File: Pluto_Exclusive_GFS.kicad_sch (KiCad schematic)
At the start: 26 parts

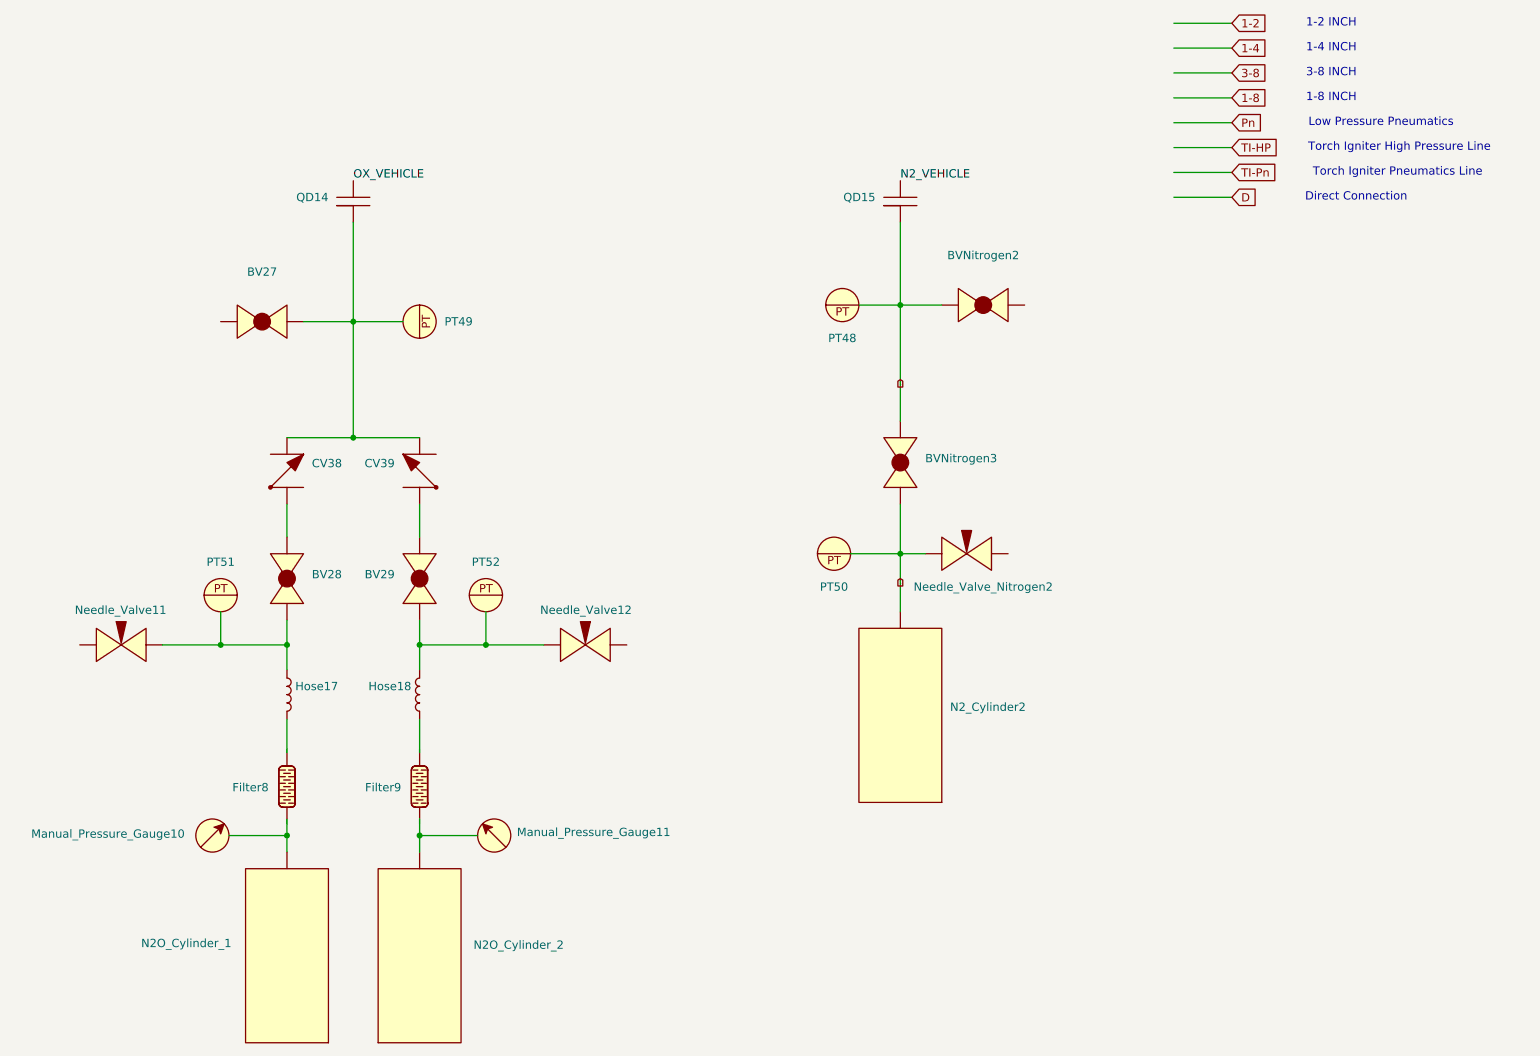
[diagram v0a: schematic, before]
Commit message: more silwood stuff
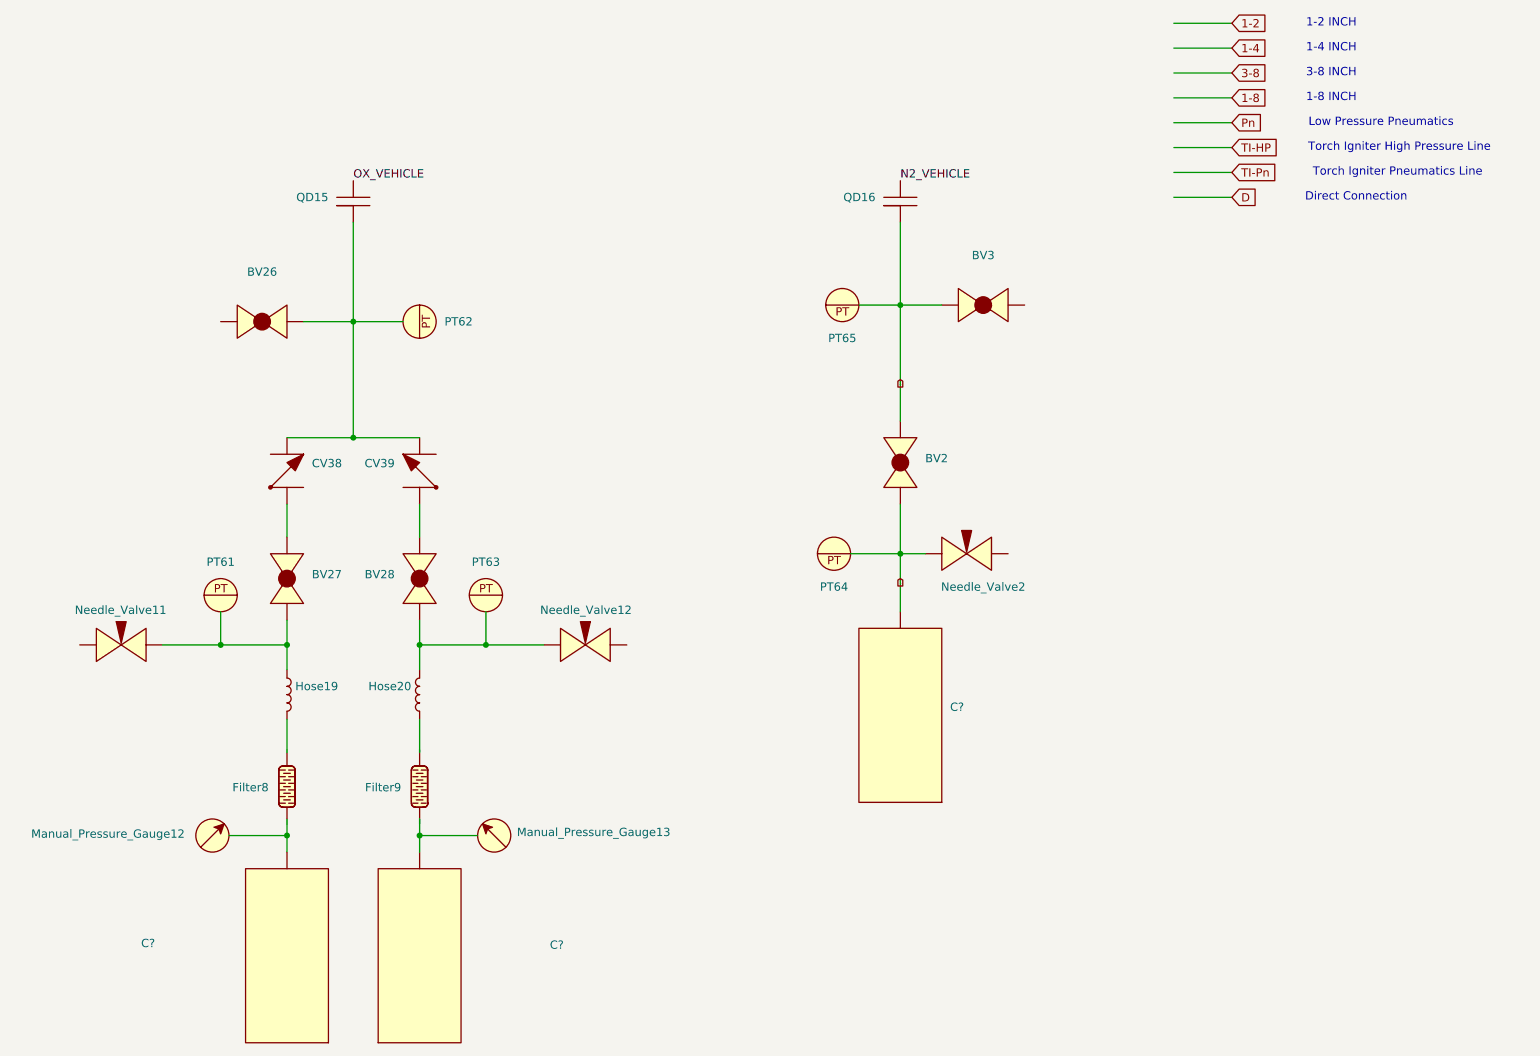
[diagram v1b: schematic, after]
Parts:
- renumbered BVNitrogen3 to BV2, BV27 to BV26, BV28 to BV27, BV29 to BV28, BVNitrogen2 to BV3, N2_Cylinder2 to C?, N2O_Cylinder_1 to C?, N2O_Cylinder_2 to C?, Hose17 to Hose19, Hose18 to Hose20, Manual_Pressure_Gauge10 to Manual_Pressure_Gauge12, Manual_Pressure_Gauge11 to Manual_Pressure_Gauge13, Needle_Valve_Nitrogen2 to Needle_Valve2, PT51 to PT61, PT49 to PT62, PT52 to PT63, PT50 to PT64, PT48 to PT65, QD14 to QD15, QD15 to QD16
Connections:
- net at Hose20.: now also BV28., Needle_Valve12., PT63.
- net at Manual_Pressure_Gauge12.: now also C?.
- net at Hose19.: now also BV27., Needle_Valve11., PT61.
- net at Manual_Pressure_Gauge13.: now also C?.
- new net: BV26., CV38., CV39., PT62., QD15.
- now unconnected: BV26., Needle_Valve11., Needle_Valve12., PT61., PT62., PT63.

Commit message: Formatiing
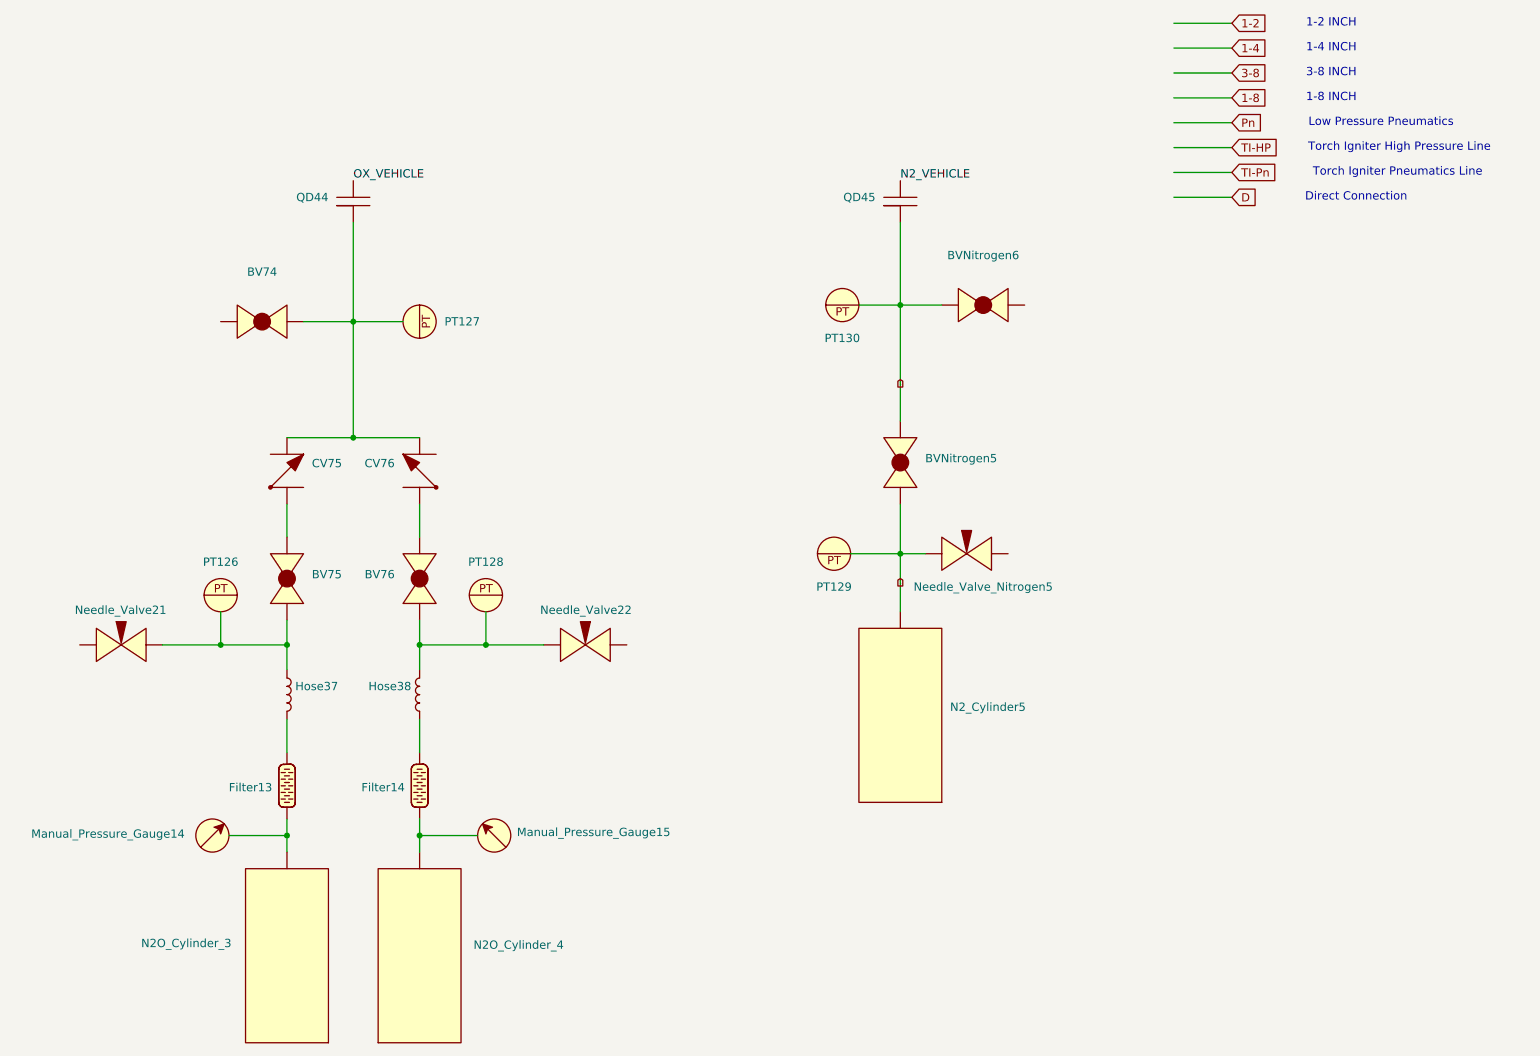
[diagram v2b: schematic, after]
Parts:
- gave numbers to parts that had none: 3
- renumbered BV26 to BV74, BV27 to BV75, BV28 to BV76, BV2 to BVNitrogen5, BV3 to BVNitrogen6, CV38 to CV75, CV39 to CV76, Filter8 to Filter13, Filter9 to Filter14, Hose19 to Hose37, Hose20 to Hose38, Manual_Pressure_Gauge12 to Manual_Pressure_Gauge14, Manual_Pressure_Gauge13 to Manual_Pressure_Gauge15, Needle_Valve11 to Needle_Valve21, Needle_Valve12 to Needle_Valve22, Needle_Valve2 to Needle_Valve_Nitrogen5, PT61 to PT126, PT62 to PT127, PT63 to PT128, PT64 to PT129, PT65 to PT130, QD15 to QD44, QD16 to QD45
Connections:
- net at Hose38.: now also BV76., Needle_Valve22., PT128.
- net at Manual_Pressure_Gauge14.: now also Filter13., N2O_Cylinder_3.
- net at Hose37.: now also Filter13.
- net at Manual_Pressure_Gauge15.: now also Filter14., N2O_Cylinder_4.
- new net: Filter14., Hose38.
- new net: BV74., CV75., CV76., PT127., QD44.
- new net: BV75., Hose37., Needle_Valve21., PT126.
- now unconnected: BV74., Needle_Valve21., Needle_Valve22., PT126., PT127., PT128.
